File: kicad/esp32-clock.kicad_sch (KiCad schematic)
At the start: 19 parts, among them J1 Conn_01x07_Socket, SW1 RESET, SW2 BOOT, U1 ESP32-PICO-V3

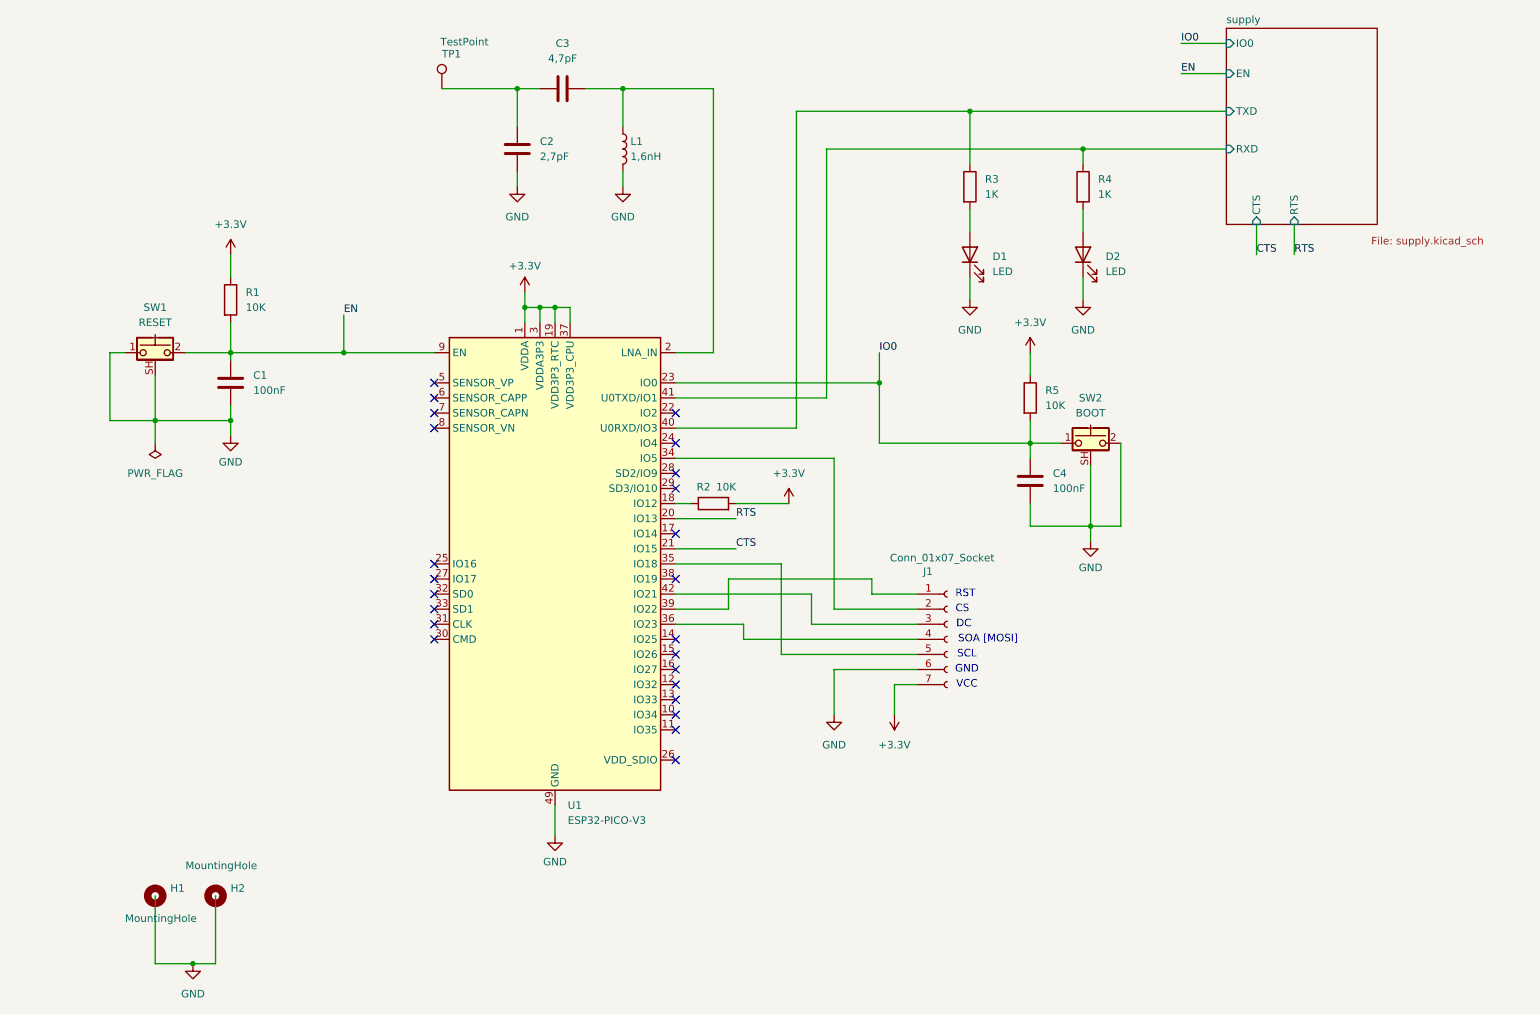
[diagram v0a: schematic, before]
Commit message: init
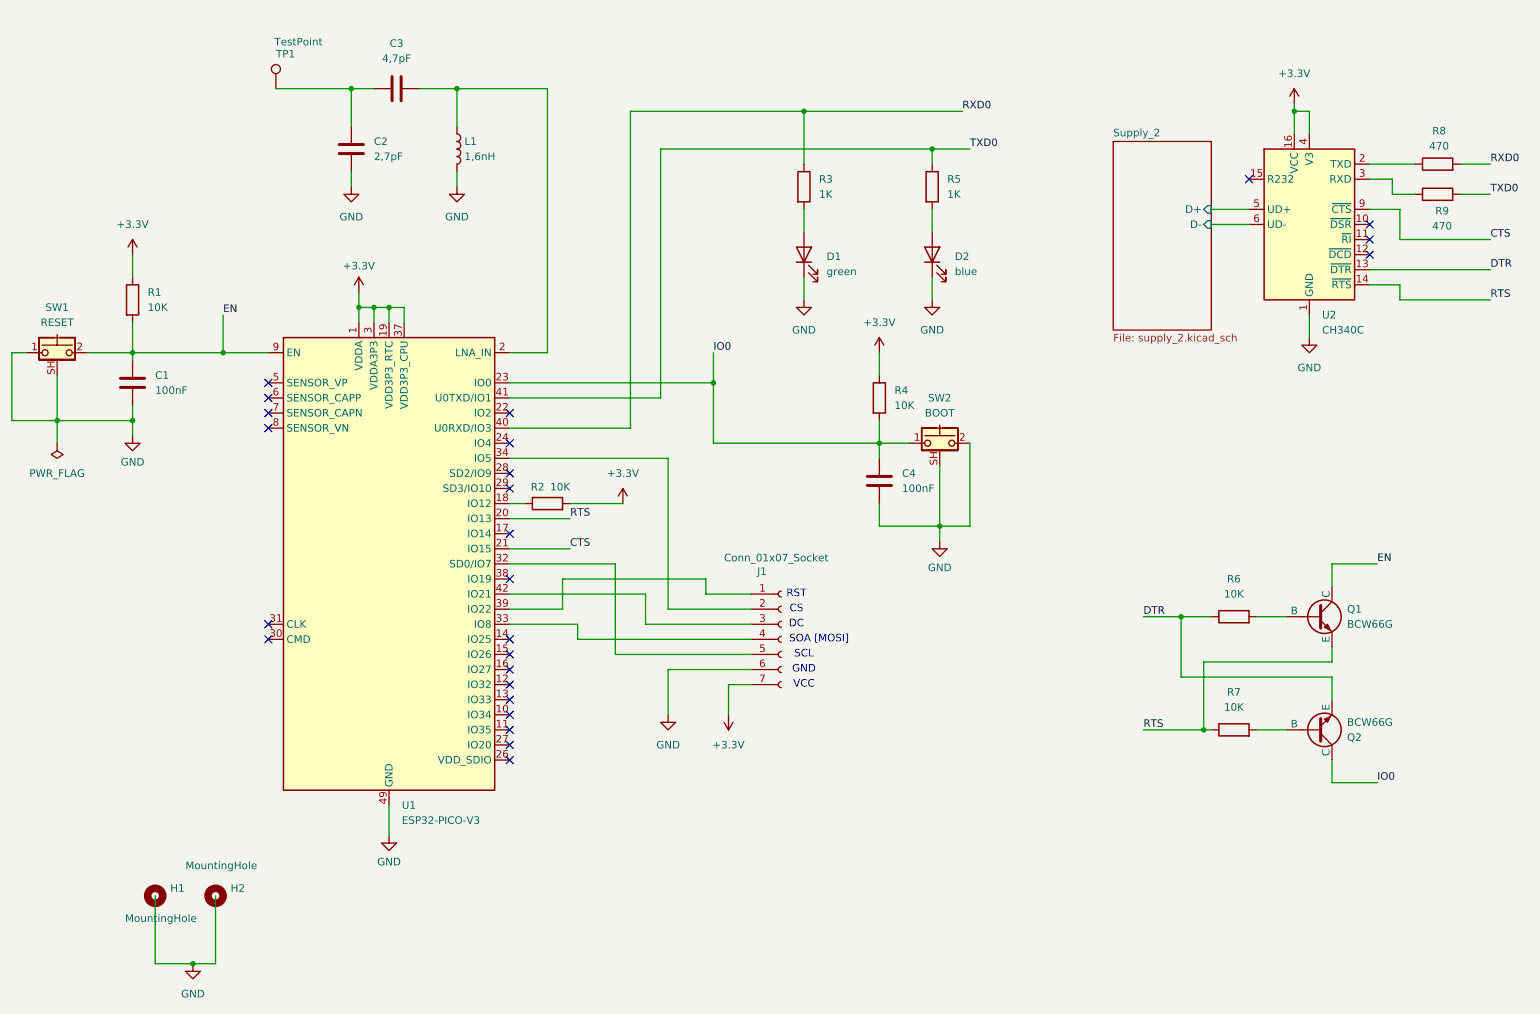
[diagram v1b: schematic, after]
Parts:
- added Q1, Q2: BCW66G, Package_TO_SOT_SMD:SOT-23, symbol Simulation_SPICE:NPN
- added R6, R7: 10K, Resistor_SMD:R_1206_3216Metric, symbol Device:R
- added R8, R9: 470, Resistor_SMD:R_1206_3216Metric, symbol Device:R
- added U2: CH340C, Package_SO:SOIC-16_3.9x9.9mm_P1.27mm, symbol Interface_USB:CH340C
- D1: value LED -> green
- D2: value LED -> blue
- renumbered R5 to R4, R4 to R5
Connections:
- net +3.3V: now also U2.16 (VCC), U2.4 (V3)
- net CTS: now also U2.9 (~{CTS})
- net EN: now also Q1.1 (C)
- net GND: now also U2.1 (GND)
- net IO0: now also Q2.1 (C)
- net RTS: now also Q1.3 (E), R7.1, U2.14 (~{RTS})
- net at J1.4 (Pin_4): now also U1.33 (IO8); no longer U1.36 (IO23)
- net at J1.5 (Pin_5): now also U1.32 (SD0/IO7); no longer U1.35 (IO18)
- net supply/RXD renamed TXD0
- net TXD0: now also R9.2
- net supply/TXD renamed RXD0
- net RXD0: now also R8.2
- new net: R8.1, U2.2 (TXD)
- new net: R9.1, U2.3 (RXD)
- new net: Q2.2 (B), R7.2
- new net: Q1.2 (B), R6.2
- new net DTR: Q2.3 (E), R6.1, U2.13 (~{DTR})
- new net Supply_2/D+: U2.5 (UD+)
- new net Supply_2/D-: U2.6 (UD-)
- no-connect marks 24 -> 25
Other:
- removed sheet supply
- added sheet Supply_2 (supply_2.kicad_sch)
- moved on the sheet: C1, C2, C3, C4, D1, D2, J1, L1, R1, R2, R3, R4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
